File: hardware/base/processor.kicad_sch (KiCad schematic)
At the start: 10 parts, among them SW1 RESET, SW2 BOOT, SW4 NAV, U6 ESP32-S3-WROOM-1

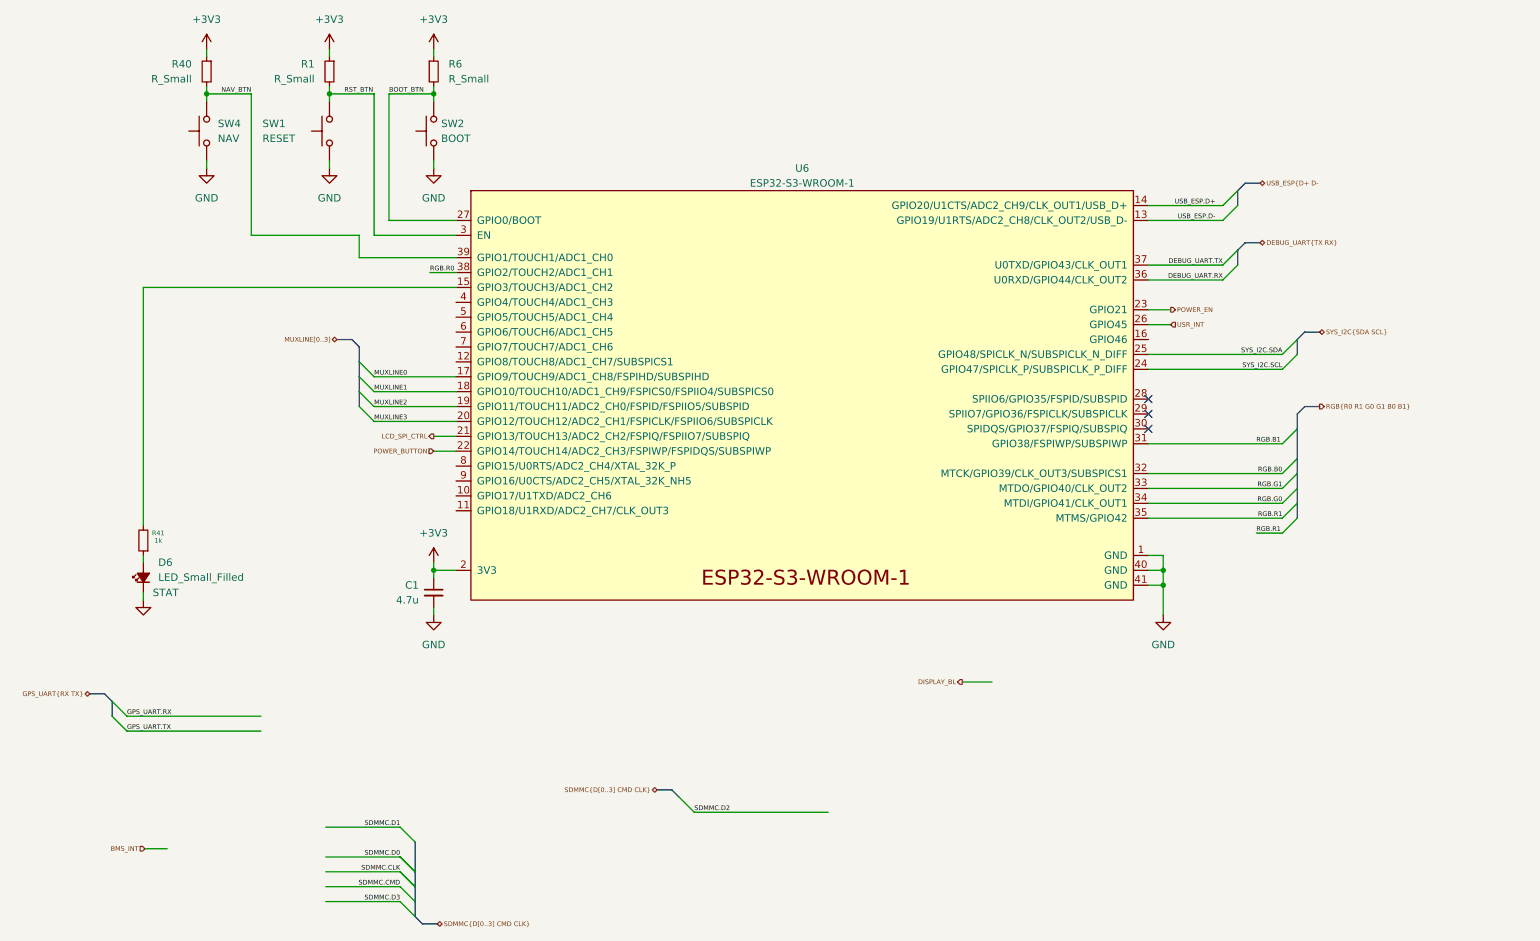
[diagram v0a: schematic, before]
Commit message: schematic complete unreviewed
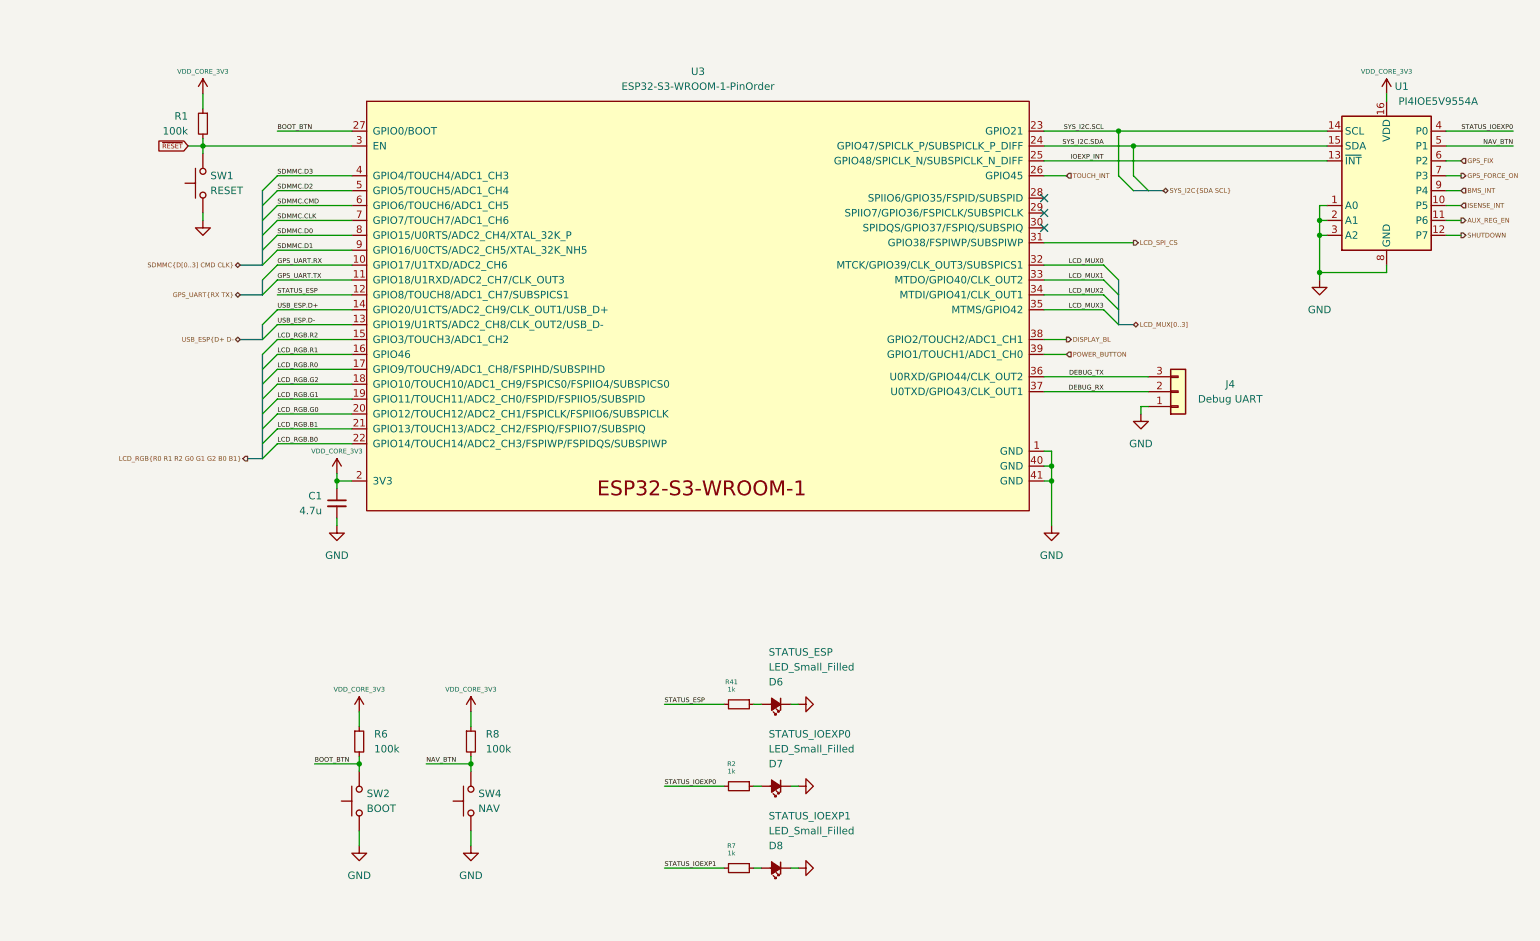
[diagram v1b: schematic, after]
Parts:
- removed R40: R_Small, Resistor_SMD:R_0402_1005Metric, symbol Device:R_Small
- removed U6: ESP32-S3-WROOM-1, bt_Espressif:ESP32-S3-WROOM-1U, symbol bt_Espressif:ESP32-S3-WROOM-1
- added D7, D8: LED_Small_Filled, LED_SMD:LED_0603_1608Metric, symbol Device:LED_Small_Filled
- added J4: Debug UART, Connector_PinHeader_2.54mm:PinHeader_1x03_P2.54mm_Vertical, symbol Connector_Generic:Conn_01x03
- added R2, R7: 1k, Resistor_SMD:R_0402_1005Metric, symbol Device:R_Small
- added R8: 100k, Resistor_SMD:R_0402_1005Metric, symbol Device:R_Small
- added U1: PI4IOE5V9554A, Package_SO:TSSOP-16_4.4x5mm_P0.65mm, symbol Interface_Expansion:TCA9554PW
- added U3: ESP32-S3-WROOM-1-PinOrder, bt_Espressif:ESP32-S3-WROOM-1U, symbol bt_Espressif:ESP32-S3-WROOM-1-PinOrder
- D6: footprint LED_SMD:LED_0402_1005Metric -> LED_SMD:LED_0603_1608Metric; Label STAT -> STATUS_ESP
- R1, R6: value R_Small -> 100k
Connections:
- net BMS_INT: now also U1.9 (P4)
- net BOOT_BTN: now also U3.27 (GPIO0/BOOT)
- net DISPLAY_BL: now also U3.38 (GPIO2/TOUCH2/ADC1_CH1)
- net GND: now also D7.1 (K), D8.1 (K), J4.1 (Pin_1), U1.1 (A0), U1.2 (A1), U1.3 (A2), U1.8 (GND), U3.1 (GND), U3.40 (GND), U3.41 (GND)
- net GPS_UART.RX: now also U3.10 (GPIO17/U1TXD/ADC2_CH6)
- net GPS_UART.TX: now also U3.11 (GPIO18/U1RXD/ADC2_CH7/CLK_OUT3)
- net NAV_BTN: now also R8.2, U1.5 (P1)
- net POWER_BUTTON: now also U3.39 (GPIO1/TOUCH1/ADC1_CH0)
- net SDMMC.CLK: now also U3.7 (GPIO7/TOUCH7/ADC1_CH6)
- net SDMMC.CMD: now also U3.6 (GPIO6/TOUCH6/ADC1_CH5)
- net SDMMC.D0: now also U3.8 (GPIO15/U0RTS/ADC2_CH4/XTAL_32K_P)
- net SDMMC.D1: now also U3.9 (GPIO16/U0CTS/ADC2_CH5/XTAL_32K_NH5)
- net SDMMC.D2: now also U3.5 (GPIO5/TOUCH5/ADC1_CH4)
- net SDMMC.D3: now also U3.4 (GPIO4/TOUCH4/ADC1_CH3)
- net SYS_I2C.SCL: now also U1.14 (SCL), U3.23 (GPIO21)
- net SYS_I2C.SDA: now also U1.15 (SDA), U3.24 (GPIO47/SPICLK_P/SUBSPICLK_P_DIFF)
- net USB_ESP.D+: now also U3.14 (GPIO20/U1CTS/ADC2_CH9/CLK_OUT1/USB_D+)
- net USB_ESP.D-: now also U3.13 (GPIO19/U1RTS/ADC2_CH8/CLK_OUT2/USB_D-)
- net STATUS_ESP: now reaches R41.2
- net STATUS_ESP: now also U3.12 (GPIO8/TOUCH8/ADC1_CH7/SUBSPICS1)
- net +3V3 renamed VDD_CORE_3V3
- net VDD_CORE_3V3: now also R8.1, U1.16 (VDD), U3.2 (3V3)
- net RST_BTN renamed ~{RESET}
- net ~{RESET}: now also U3.3 (EN)
- new net: D7.2 (A), R2.1
- new net: D8.2 (A), R7.1
- new net AUX_REG_EN: U1.11 (P6)
- new net DEBUG_RX: J4.2 (Pin_2), U3.37 (U0TXD/GPIO43/CLK_OUT1)
- new net DEBUG_TX: J4.3 (Pin_3), U3.36 (U0RXD/GPIO44/CLK_OUT2)
- new net GPS_FIX: U1.6 (P2)
- new net GPS_FORCE_ON: U1.7 (P3)
- new net IOEXP_INT: U1.13 (~{INT}), U3.25 (GPIO48/SPICLK_N/SUBSPICLK_N_DIFF)
- new net ISENSE_INT: U1.10 (P5)
- new net LCD_MUX0: U3.32 (MTCK/GPIO39/CLK_OUT3/SUBSPICS1)
- new net LCD_MUX1: U3.33 (MTDO/GPIO40/CLK_OUT2)
- new net LCD_MUX2: U3.34 (MTDI/GPIO41/CLK_OUT1)
- new net LCD_MUX3: U3.35 (MTMS/GPIO42)
- new net LCD_RGB.B0: U3.22 (GPIO14/TOUCH14/ADC2_CH3/FSPIWP/FSPIDQS/SUBSPIWP)
- new net LCD_RGB.B1: U3.21 (GPIO13/TOUCH13/ADC2_CH2/FSPIQ/FSPIIO7/SUBSPIQ)
- new net LCD_RGB.G0: U3.20 (GPIO12/TOUCH12/ADC2_CH1/FSPICLK/FSPIIO6/SUBSPICLK)
- new net LCD_RGB.G1: U3.19 (GPIO11/TOUCH11/ADC2_CH0/FSPID/FSPIIO5/SUBSPID)
- new net LCD_RGB.G2: U3.18 (GPIO10/TOUCH10/ADC1_CH9/FSPICS0/FSPIIO4/SUBSPICS0)
- new net LCD_RGB.R0: U3.17 (GPIO9/TOUCH9/ADC1_CH8/FSPIHD/SUBSPIHD)
- new net LCD_RGB.R1: U3.16 (GPIO46)
- new net LCD_RGB.R2: U3.15 (GPIO3/TOUCH3/ADC1_CH2)
- new net LCD_SPI_CS: U3.31 (GPIO38/FSPIWP/SUBSPIWP)
- new net SHUTDOWN: U1.12 (P7)
- new net STATUS_IOEXP0: R2.2, U1.4 (P0)
- new net STATUS_IOEXP1: R7.2
- new net TOUCH_INT: U3.26 (GPIO45)
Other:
- moved on the sheet: C1, D6, R1, R41, R6, SW1, SW2
